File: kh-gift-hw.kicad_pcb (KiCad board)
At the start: 2 copper layers, 49.4 x 55 mm, 34 parts, among them J1 Conn_01x02, J2 Conn_01x06, J3 Conn_01x03, J4 Conn_01x14, Q1 MMBT5550, SW1 SW_Push, SW2 SW_Push, U1 ESP32-WROVER, U2 AMS1117-3.3, U3 DHT11, U4 DS1307Z+, Y1 Crystal

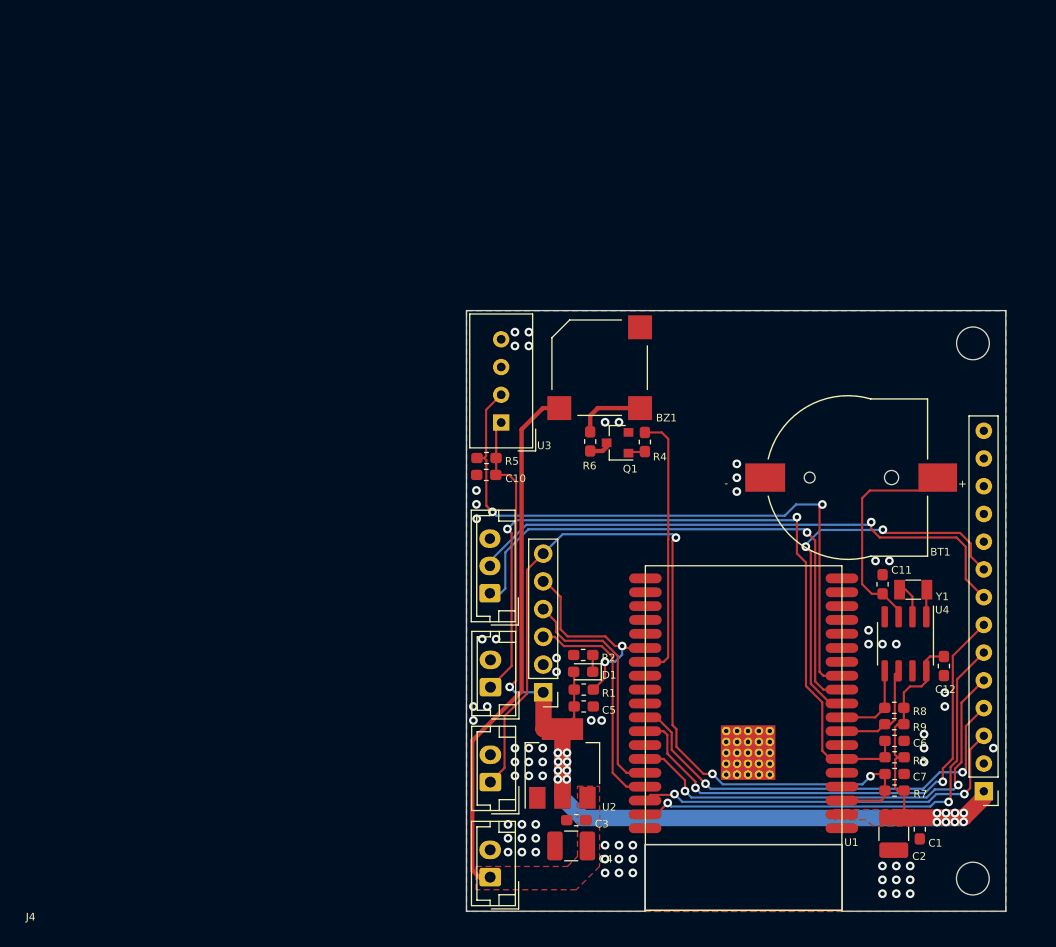
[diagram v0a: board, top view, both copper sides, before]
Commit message: update routing
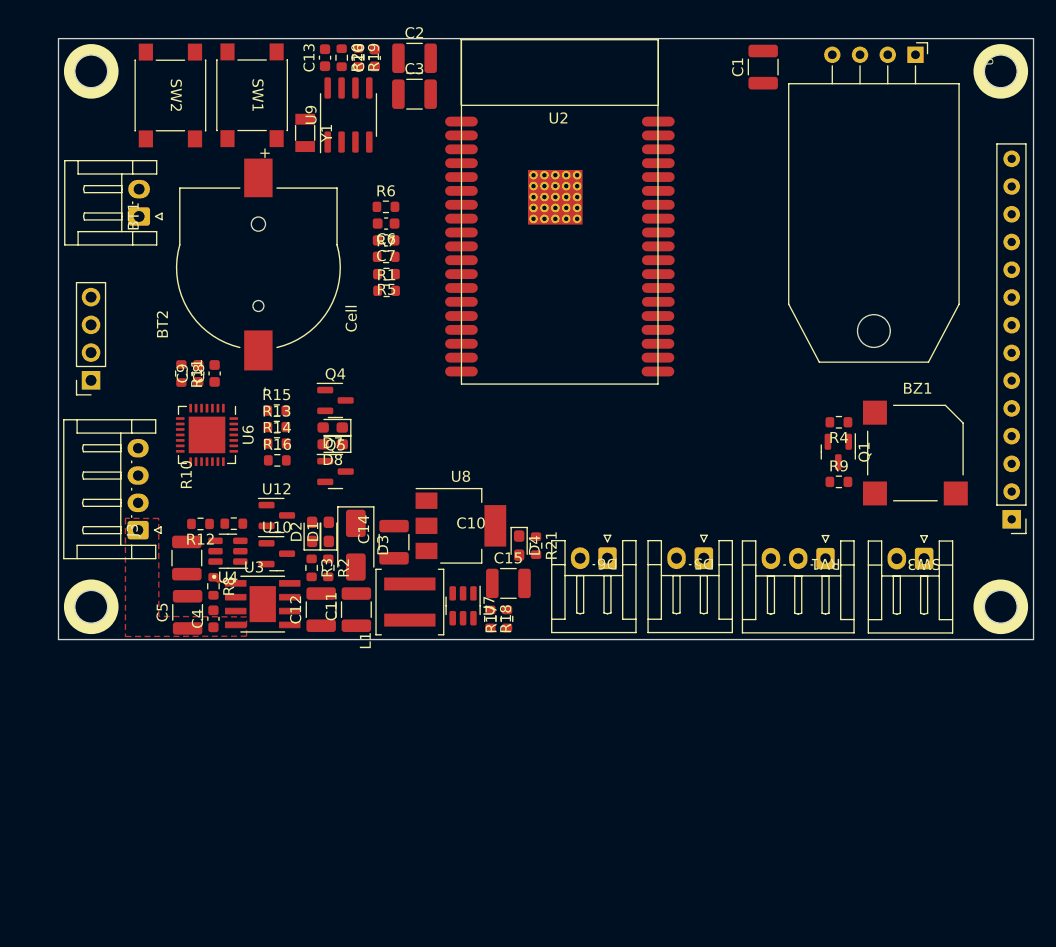
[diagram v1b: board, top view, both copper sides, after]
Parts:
- removed J1: Conn_01x02, Connector_JST:JST_EH_B2B-EH-A_1x02_P2.50mm_Vertical
- removed J4: Conn_01x14, footprints:ili9341_3.2inch
- added BT2: Cell, footprints:BAT_CR1220_Holder, F.Cu at (50.8, 113.5)
- added C13: 100nF, Capacitor_SMD:C_0603_1608Metric, F.Cu at (56.9, 94.2)
- added C14: 10uF, Capacitor_SMD:C_1210_3225Metric, F.Cu at (63.2, 138.6)
- added C15: 10uF, Capacitor_SMD:C_1210_3225Metric, F.Cu at (73.7, 142.4)
- added C16: 100nF, Capacitor_SMD:C_0603_1608Metric, F.Cu at (61.4, 94.3)
- added C8: 100nF, Capacitor_SMD:C_0603_1608Metric, F.Cu at (46.8, 123.2)
- added C9: 10uF, Capacitor_SMD:C_0603_1608Metric, F.Cu at (45.3, 123.2)
- added D2: RED, LED_SMD:LED_0603_1608Metric_Pad1.05x0.95mm_HandSolder, F.Cu at (55.7, 137.7)
- added D3: SS24, Diode_SMD:D_SMA, F.Cu at (59.7, 138.9)
- added D4: YELLOW, LED_SMD:LED_0603_1608Metric_Pad1.05x0.95mm_HandSolder, F.Cu at (74.7, 138.9)
- added D5: GREEN, footprints:JST_EH_S2B-EH_1x02_P2.5mm_Horizontal, F.Cu at (91.6, 140.1)
- added D6: RED, footprints:JST_EH_S2B-EH_1x02_P2.5mm_Horizontal, F.Cu at (82.8, 140.1)
- added D7: TX, LED_SMD:LED_0603_1608Metric_Pad1.05x0.95mm_HandSolder, F.Cu at (57.6, 128.1)
- added D8: RX, LED_SMD:LED_0603_1608Metric_Pad1.05x0.95mm_HandSolder, F.Cu at (57.6, 129.7)
- added L1: 0.1H, Inductor_SMD:L_Coilcraft_XAL5030-XXX, F.Cu at (64.7, 144.1)
- added Q4: MMBT2222A, Package_TO_SOT_SMD:SOT-23, F.Cu at (57.9, 125.6)
- added Q5: MMBT2222A, Package_TO_SOT_SMD:SOT-23, F.Cu at (57.9, 132.1)
- added R10: 1k, Resistor_SMD:R_0603_1608Metric, F.Cu at (48.5, 136.9)
- added R11: 10k, Resistor_SMD:R_0603_1608Metric, F.Cu at (43.7, 123.2)
- added R12: 100R, Resistor_SMD:R_0603_1608Metric, F.Cu at (45.5, 136.9)
- added R13: 330R, Resistor_SMD:R_0603_1608Metric, F.Cu at (52.5, 128.1)
- added R14: 330R, Resistor_SMD:R_0603_1608Metric, F.Cu at (52.5, 129.6)
- added R15: 10k, Resistor_SMD:R_0603_1608Metric, F.Cu at (52.5, 126.6)
- added R16: 10k, Resistor_SMD:R_0603_1608Metric, F.Cu at (52.5, 131.1)
- added R17: TBD, Resistor_SMD:R_0603_1608Metric, F.Cu at (73.6, 145.6)
- added R18: TBD, Resistor_SMD:R_0603_1608Metric, F.Cu at (72.0, 145.6)
- added R19: 4K7, Resistor_SMD:R_0603_1608Metric, F.Cu at (59.9, 94.2)
- added R20: 4K7, Resistor_SMD:R_0603_1608Metric, F.Cu at (58.4, 94.2)
- added R21: 330R, Resistor_SMD:R_0603_1608Metric, F.Cu at (76.2, 138.9)
- added RV1: Potentiometer, footprints:JST_EH_S3B-EH_1x03_P2.5mm_Horizontal, F.Cu at (102.7, 140.1)
- added SW3: SW_Push, footprints:JST_EH_S2B-EH_1x02_P2.5mm_Horizontal, F.Cu at (111.8, 140.1)
- added U10: IRLML0030, Package_TO_SOT_SMD:SOT-23, F.Cu at (52.5, 139.7)
- added U12: IRLML0030, Package_TO_SOT_SMD:SOT-23, F.Cu at (52.5, 136.2)
- added U6: CP2102N-Axx-xQFN28, Package_DFN_QFN:QFN-28-1EP_5x5mm_P0.5mm_EP3.35x3.35mm, F.Cu at (46.1, 128.8)
- added U7: SX1308, Package_TO_SOT_SMD:TSOT-23-6, F.Cu at (69.5, 144.4)
- added U8: AMS1117-3.3, Package_TO_SOT_SMD:SOT-223-3_TabPin2, F.Cu at (69.3, 137.1)
- added U9: DS1307Z+, Package_SO:SOIC-8_3.9x4.9mm_P1.27mm, F.Cu at (59.0, 99.5)
- BT1: value Battery_Cell -> PinLipo; footprint footprints:BAT_CR1220_Holder -> footprints:JST_EH_S2B-EH_1x02_P2.5mm_Horizontal
- C1: footprint Capacitor_SMD:C_0603_1608Metric_Pad1.05x0.95mm_HandSolder -> Capacitor_SMD:C_1210_3225Metric
- C10: value 100nF -> 0.1uF; footprint Capacitor_SMD:C_0603_1608Metric_Pad1.05x0.95mm_HandSolder -> Capacitor_SMD:C_1210_3225Metric
- C11, C12, C3, C5: value 100nF -> 10uF; footprint Capacitor_SMD:C_0603_1608Metric_Pad1.05x0.95mm_HandSolder -> Capacitor_SMD:C_1210_3225Metric
- C2: value 10uF -> 100nF; footprint Capacitor_SMD:C_1210_3225Metric_Pad1.42x2.65mm_HandSolder -> Capacitor_SMD:C_1210_3225Metric
- C4: value 10uF -> 100nF; footprint Capacitor_SMD:C_1210_3225Metric_Pad1.42x2.65mm_HandSolder -> Capacitor_SMD:C_0603_1608Metric
- C6, C7: footprint Capacitor_SMD:C_0603_1608Metric_Pad1.05x0.95mm_HandSolder -> Capacitor_SMD:C_0603_1608Metric
- D1: value LED_Small -> GREEN
- J2: value Conn_01x06 -> Conn_01x14; footprint Connector_PinHeader_2.54mm:PinHeader_1x06_P2.54mm_Vertical -> footprints:ili9341_3.2inch
- J3: value Conn_01x03 -> USB; footprint Connector_JST:JST_EH_B3B-EH-A_1x03_P2.50mm_Vertical -> footprints:JST_EH_S4B-EH_1x04_P2.5mm_Horizontal
- R1: value 10K -> NC; footprint Resistor_SMD:R_0603_1608Metric_Pad1.05x0.95mm_HandSolder -> Resistor_SMD:R_0603_1608Metric
- R2: value 330R -> 1k; footprint Resistor_SMD:R_0603_1608Metric_Pad1.05x0.95mm_HandSolder -> Resistor_SMD:R_0603_1608Metric
- R3: value 10K -> 1k; footprint Resistor_SMD:R_0603_1608Metric_Pad1.05x0.95mm_HandSolder -> Resistor_SMD:R_0603_1608Metric
- R4, R7: footprint Resistor_SMD:R_0603_1608Metric_Pad1.05x0.95mm_HandSolder -> Resistor_SMD:R_0603_1608Metric
- R5: value NC -> 10K; footprint Resistor_SMD:R_0603_1608Metric_Pad1.05x0.95mm_HandSolder -> Resistor_SMD:R_0603_1608Metric
- R6: value 0R -> 10K; footprint Resistor_SMD:R_0603_1608Metric_Pad1.05x0.95mm_HandSolder -> Resistor_SMD:R_0603_1608Metric
- R8: value 4K7 -> 1.2k; footprint Resistor_SMD:R_0603_1608Metric_Pad1.05x0.95mm_HandSolder -> Resistor_SMD:R_0603_1608Metric
- R9: value 4K7 -> 0R; footprint Resistor_SMD:R_0603_1608Metric_Pad1.05x0.95mm_HandSolder -> Resistor_SMD:R_0603_1608Metric
- SW1, SW2: footprint Connector_JST:JST_EH_B2B-EH-A_1x02_P2.50mm_Vertical -> footprints:PushButton_6x6mm_SMD
- U1: value ESP32-WROVER -> DHT11; footprint footprints:ESP32-WROVER -> footprints:SNR4-2.54-15.5X12.0X5.5MM
- U2: value AMS1117-3.3 -> ESP32-WROVER; footprint Package_TO_SOT_SMD:SOT-223-3_TabPin2 -> footprints:ESP32-WROVER
- U3: value DHT11 -> TP4056; footprint Sensor:Aosong_DHT11_5.5x12.0_P2.54mm -> footprints:SOP127P600X175-9N
- U4: value DS1307Z+ -> DW01A; footprint Package_SO:SOIC-8_3.9x4.9mm_P1.27mm -> Package_TO_SOT_SMD:TSOT-23-6
- Y1: value Crystal -> 32768 kHz
- moved C2 83.5 mm to (65.1, 94.3), turned to 0 degrees
- moved U1 73.5 mm to (111.0, 94.0), turned to -90 degrees
- moved C1 71.3 mm to (97.0, 95.1), turned to 90 degrees
- moved Y1 69.7 mm to (55.1, 101.1), turned to -90 degrees
- moved SW2 69.4 mm to (42.7, 97.7), turned to -90 degrees
- moved BT1 69.2 mm to (39.9, 108.8), turned to 90 degrees
- moved C3 68.1 mm to (65.1, 97.6), turned to 0 degrees
- moved C7 67.5 mm to (62.5, 111.0), turned to 180 degrees
- moved R7 67.5 mm to (62.5, 112.5), turned to 0 degrees
- moved C6 66.4 mm to (62.5, 109.4), turned to 180 degrees
- moved R8 63.3 mm to (46.7, 142.7), turned to -90 degrees
- moved U4 62.6 mm to (48.0, 139.4), turned to 180 degrees
- moved U2 59.7 mm to (78.4, 99.2), turned to 0 degrees
- moved SW1 58.4 mm to (50.2, 97.7), turned to -90 degrees
- moved C12 57.3 mm to (56.5, 144.8), turned to 90 degrees
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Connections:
- BT1 pad 1: VBAT -> Net-(BT1-+)
- BT1 pad 2: GND -> Net-(BT1--)
- BZ1 pad 2: Net-(BZ1-Pad2) -> Net-(BZ1-+)
- C10 pad 1: +3V3 -> Net-(U4-VCC)
- C10 pad 2: GND -> Net-(BT1--)
- C11 pad 1: VBAT -> Net-(BT1-+)
- C12 pad 1: +3V3 -> Net-(BT1-+)
- C3 pad 1: +5V -> +3V3
- C4 pad 1: +5V -> 5V_USB
- C5 pad 1: +3V3 -> 5V_USB
- C6 pad 1: BUTTON -> FLASH_EN
- C7 pad 1: FLASH_EN -> BUTTON
- D1 pad 2: +3V3 -> 5V_USB
- J2 pad 3: FLASH_U0TX -> LCD_CS
- J2 pad 4: FLASH_U0RX -> LCD_RST
- J2 pad 5: FLASH_IO0 -> LCD_DC
- J2 pad 6: FLASH_EN -> LCD_MOSI
- J3 pad 1: LCD_BCKL -> 5V_USB
- J3 pad 2: Net-(J3-Pad2) -> CP2102_D+
- J3 pad 3: GND -> CP2102_D-
- Q1 pad 3: Net-(Q1-Pad3) -> Net-(Q1-C)
- R1 pad 1: FLASH_IO0 -> +3V3
- R1 pad 2: +3V3 -> DHT
- R2 pad 2: GND -> Net-(U3-STDBY)
- R3 pad 1: +3V3 -> Net-(D2-K)
- R3 pad 2: BUTTON -> Net-(U3-CHRG)
- R5 pad 1: +3V3 -> FLASH_IO0
- R5 pad 2: DHT -> +3V3
- R6 pad 1: Net-(BZ1-Pad2) -> +3V3
- R6 pad 2: Net-(Q1-Pad3) -> FLASH_EN
- R7 pad 2: FLASH_EN -> BUTTON
- R8 pad 1: +3V3 -> Net-(U3-TEMP)
- R8 pad 2: ESP32_SDA -> GND
- R9 pad 1: +3V3 -> Net-(Q1-C)
- R9 pad 2: ESP32_SCL -> Net-(BZ1-+)
- SW1 pad 1: BUTTON -> FLASH_EN
- SW2 pad 1: FLASH_EN -> BUTTON
- U1 pad 1: GND -> +3V3
- U1 pad 2: +3V3 -> DHT
- U1 pad 3: FLASH_EN -> unconnected-(U1-NC-Pad3)
- U1 pad 4: (no net) -> GND
- U2 pad 3: +5V -> FLASH_EN
- U3 pad 1: +3V3 -> Net-(U3-TEMP)
- U3 pad 2: DHT -> GND
- U3 pad 3: (no net) -> GND
- U3 pad 4: GND -> 5V_USB
- U4 pad 1: Net-(U4-Pad1) -> Net-(U10-G)
- U4 pad 2: Net-(U4-Pad2) -> Net-(U4-VM)
- U4 pad 3: VBAT -> Net-(U12-G)
- U4 pad 4: GND -> unconnected-(U4-TD-Pad4)
- U4 pad 5: ESP32_SDA -> Net-(U4-VCC)
- U4 pad 6: ESP32_SCL -> Net-(BT1--)
- Y1 pad 1: Net-(U4-Pad1) -> Net-(U9-X1)
- Y1 pad 2: Net-(U4-Pad2) -> Net-(U9-X2)
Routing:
- net +3V3: track 117.6 -> 0.00 mm, vias 17 -> 0
- net FLASH_EN: track 82.5 -> 0.00 mm, vias 3 -> 0
- net BUTTON: track 72.4 -> 0.00 mm, vias 2 -> 0
- net DHT: track 60.8 -> 0.00 mm, vias 2 -> 0
- net Net-(J3-Pad2): track 52.0 -> 0.00 mm, vias 1 -> 0
- net LCD_BCKL: track 50.3 -> 0.00 mm, vias 1 -> 0
- net +5V: track 48.4 -> 0.00 mm
- net LCD_CLK: track 47.3 -> 0.00 mm, vias 2 -> 0
- net LCD_MOSI: track 43.6 -> 0.00 mm, vias 2 -> 0
- net LCD_DC: track 42.0 -> 0.00 mm, vias 2 -> 0
- net LCD_RST: track 40.0 -> 0.00 mm, vias 2 -> 0
- net LCD_CS: track 36.1 -> 0.00 mm, vias 2 -> 0
- net LCD_MISO: track 35.6 -> 0.00 mm, vias 2 -> 0
- net BUZZER: track 24.7 -> 0.00 mm
- net FLASH_U0RX: track 21.9 -> 0.00 mm
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- added copper zone on F.Cu, net 5V_USB
- removed copper zone on F.Cu, net +3V3
- removed copper zone on F.Cu, net +5V
- removed copper zone on B.Cu, net GND
- removed copper zone on F.Cu, net GND
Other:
- board size 49.4 x 55 mm -> 89.3 x 55 mm
- net class Default removed

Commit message: update pcb
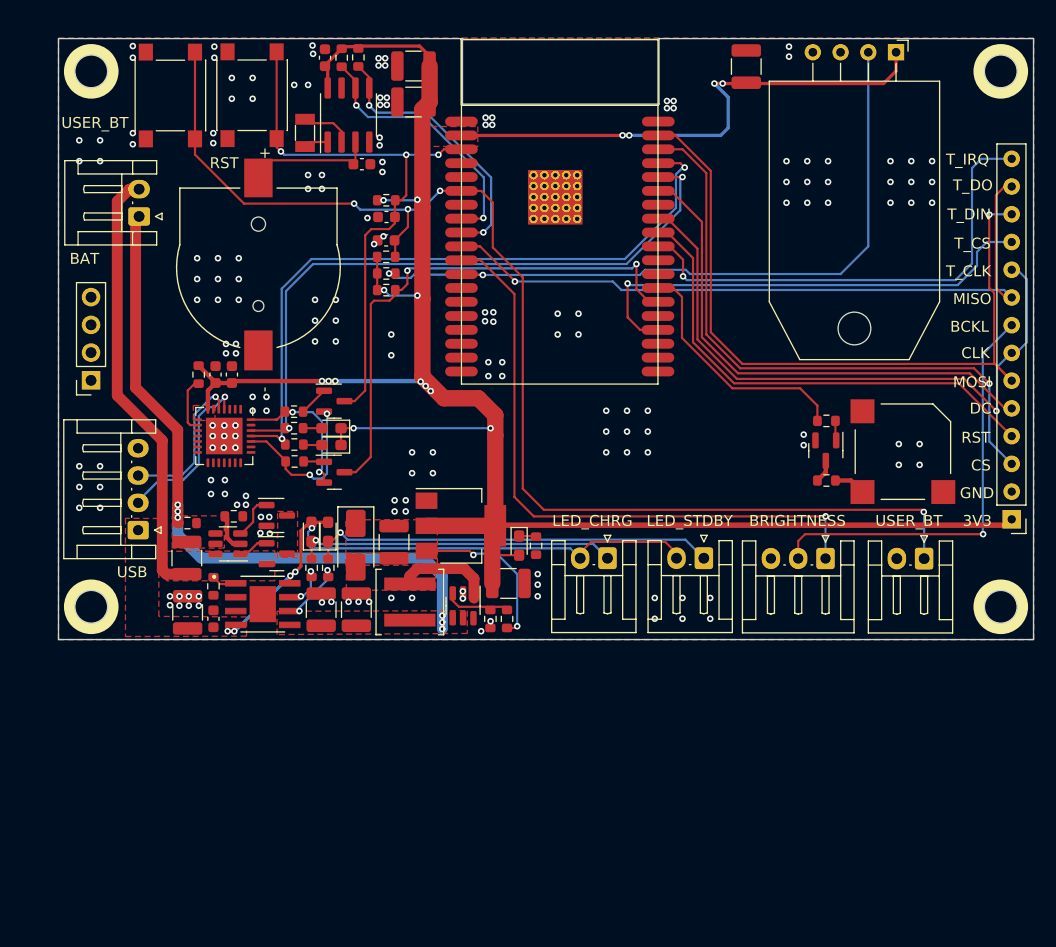
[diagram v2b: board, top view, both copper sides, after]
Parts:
- Y1: footprint Crystal:Crystal_SMD_3215-2Pin_3.2x1.5mm -> footprints:Crystal_SMD_3215-2Pin_3.2x1.5mm
- moved C16 9.80 mm to (60.3, 104.0), turned to 0 degrees
- moved U1 1.80 mm to (109.2, 93.7)
- moved R1 1.59 mm to (62.5, 114.0)
- moved R13 1.59 mm to (54.1, 128.2)
- moved R15 1.59 mm to (54.1, 126.7)
- moved C8 1.59 mm to (48.4, 123.3)
- moved C9 1.59 mm to (46.9, 123.3)
- moved R14 1.59 mm to (54.1, 129.7)
- moved R11 1.59 mm to (45.3, 123.3)
- moved R16 1.59 mm to (54.1, 131.2)
- moved U6 1.59 mm to (47.7, 128.9)
- moved C1 1.55 mm to (95.5, 95.1)
- moved R5 1.47 mm to (62.5, 115.5)
- moved R12 1.20 mm to (44.3, 136.9)
- moved BZ1 1.15 mm to (109.8, 130.3)
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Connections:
- J2 pad 10: unconnected-(J2-Pin_10-Pad10) -> LCD_CLK
- J2 pad 11: unconnected-(J2-Pin_11-Pad11) -> TOUCH_CS
- J2 pad 12: unconnected-(J2-Pin_12-Pad12) -> LCD_MOSI
- J2 pad 13: unconnected-(J2-Pin_13-Pad13) -> LCD_MISO
- J2 pad 14: unconnected-(J2-Pin_14-Pad14) -> TOUCH_IRQ
- U2 pad 23: unconnected-(U2-IO15-Pad23) -> TOUCH_CS
- U2 pad 29: unconnected-(U2-IO5-Pad29) -> TOUCH_IRQ
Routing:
- net +3V3: track 0.00 -> 224.3 mm, vias 0 -> 16
- net BUTTON: track 0.00 -> 114.1 mm, vias 0 -> 4
- net LCD_MOSI: track 0.00 -> 68.5 mm, vias 0 -> 1
- net DHT: track 0.00 -> 66.0 mm, vias 0 -> 2
- net LCD_MISO: track 0.00 -> 64.4 mm, vias 0 -> 1
- net CP2102_RX: track 0.00 -> 63.8 mm, vias 0 -> 2
- net Net-(BT1-+): track 0.00 -> 63.2 mm, vias 0 -> 6
- net CP2102_TX: track 0.00 -> 60.8 mm, vias 0 -> 2
- net LCD_CLK: track 0.00 -> 58.4 mm, vias 0 -> 1
- net LCD_BCKL: track 0.00 -> 57.8 mm, vias 0 -> 1
- net LCD_CS: track 0.00 -> 56.1 mm, vias 0 -> 1
- net 5V_USB: track 0.00 -> 55.0 mm, vias 0 -> 5
- net FLASH_EN: track 0.00 -> 52.9 mm, vias 0 -> 3
- net FLASH_IO0: track 0.00 -> 48.6 mm, vias 0 -> 2
- net LCD_DC: track 0.00 -> 46.8 mm
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- added copper zone on F.Cu, net +3V3
- added copper zone on B.Cu, net GND
- added copper zone on F.Cu, net GND
- added copper zone on F.Cu, net Net-(BT1-+)
- added copper zone on F.Cu, net Net-(BT1--)
- added copper zone on F.Cu, net Net-(D3-A)
- added copper zone on F.Cu, net Net-(D3-K)
- added copper zone on F.Cu, net Net-(U10-D)
- added copper zone on F.Cu, net Net-(U4-VCC)
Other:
- outline, holes or cut-outs redrawn
- board text added: "3V3"
- board text added: "BAT"
- board text added: "BCKL"
- board text added: "BRIGHTNESS"
- board text added: "CLK"
- board text added: "CS"
- board text added: "DC"
- board text added: "GND"
- board text added: "LED_CHRG"
- board text added: "LED_STDBY"
- board text added: "MISO"
- board text added: "MOSI"
- board text added: "RST"
- board text added: "T_CLK"
- board text added: "T_CS"
- board text added: "T_DIN"
- board text added: "T_DO"
- board text added: "T_IRQ"
- board text added: "USB"
- board text added: "USER_BT"
